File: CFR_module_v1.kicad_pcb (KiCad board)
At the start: 2 copper layers, 51 parts, among them J1 Conn_01x20, J2 Conn_01x20

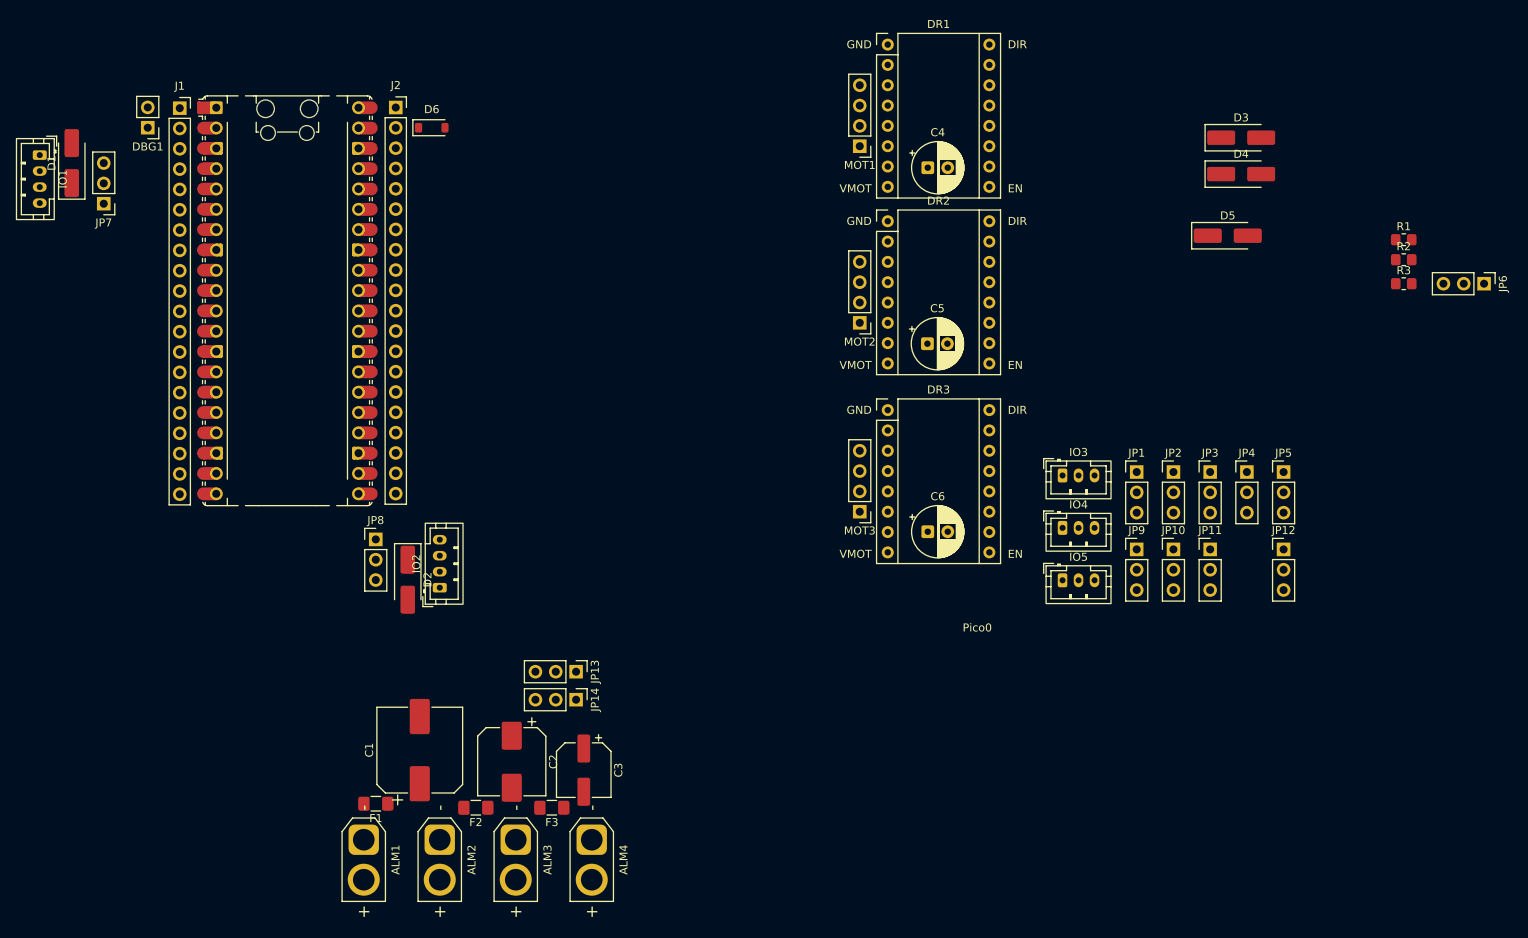
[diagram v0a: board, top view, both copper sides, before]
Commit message: pcb ok
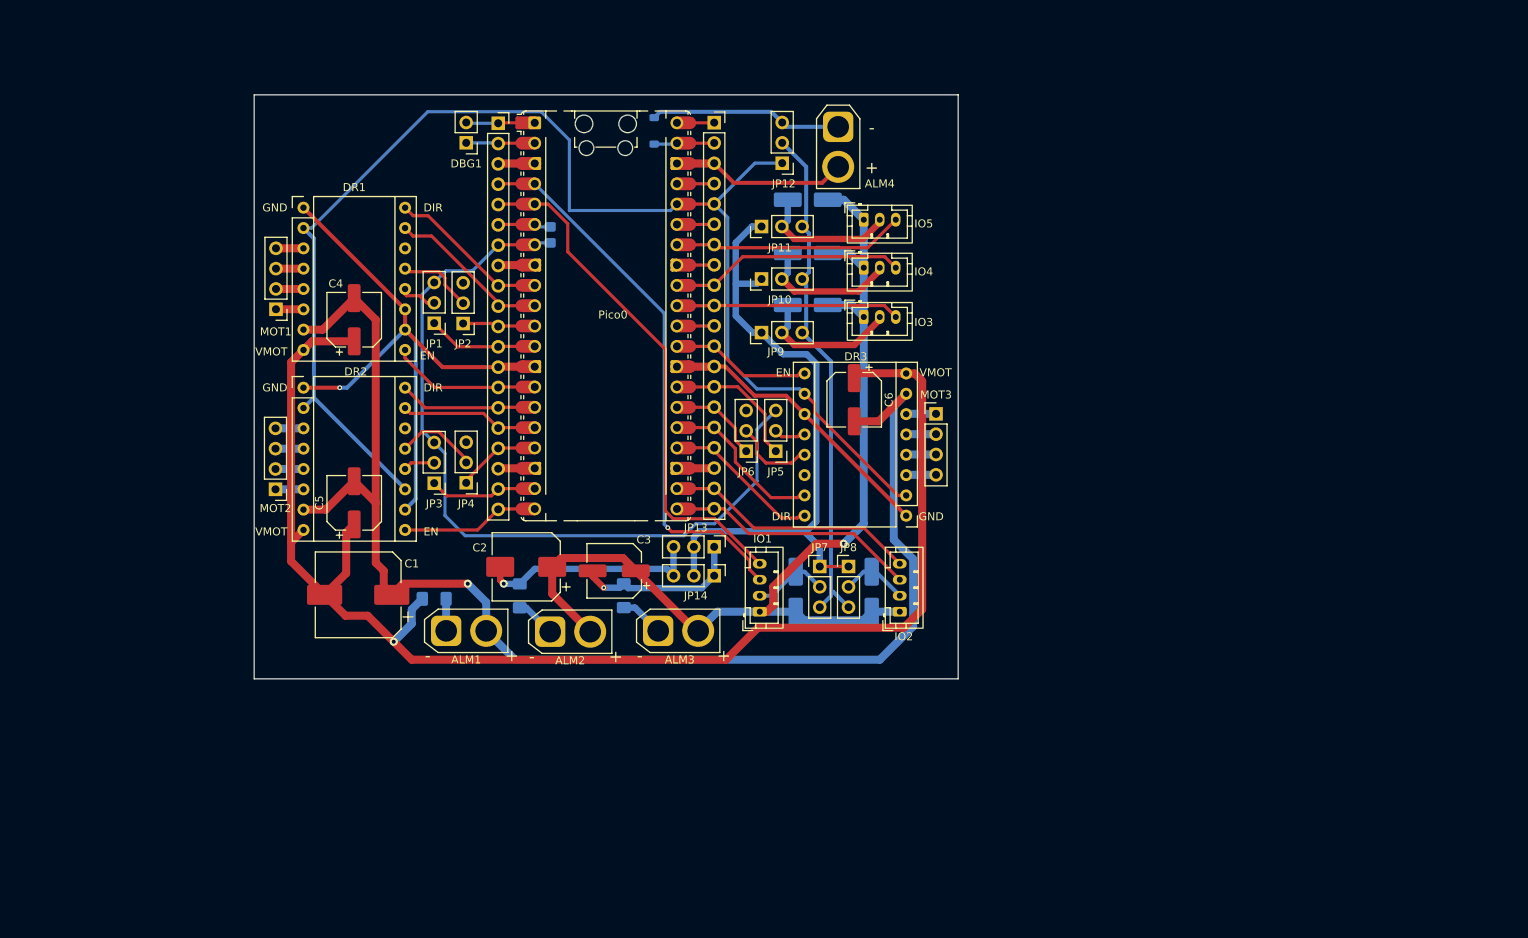
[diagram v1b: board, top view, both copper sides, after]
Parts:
- removed R2, R3: 1k, Resistor_SMD:R_0805_2012Metric_Pad1.20x1.40mm_HandSolder
- C4, C5, C6: footprint Capacitor_THT:CP_Radial_D6.3mm_P2.50mm -> Capacitor_SMD:CP_Elec_6.3x7.7
- D1, D2, D3, D4, D5, D6, F1, F2, F3, R1: moved to B.Cu
- moved R1 106.7 mm to (100.3, 83.4), turned to -90 degrees
- moved IO1 106.6 mm to (126.5, 130.5), turned to 90 degrees
- moved D1 105.2 mm to (131.0, 128.0), turned to -90 degrees
- moved JP7 100.3 mm to (134.0, 124.8), turned to 0 degrees
- moved JP4 97.6 mm to (89.8, 114.4), turned to 180 degrees
- moved JP3 97.0 mm to (85.8, 114.4), turned to 180 degrees
- moved JP6 94.6 mm to (124.8, 110.4), turned to 180 degrees
- moved ALM4 94.3 mm to (136.3, 69.9)
- moved JP2 90.7 mm to (89.4, 94.5), turned to 180 degrees
- moved JP1 89.8 mm to (85.8, 94.4), turned to 180 degrees
- moved JP12 79.1 mm to (129.3, 74.4), turned to 180 degrees
- moved DR2 75.9 mm to (69.5, 102.5)
- moved MOT2 75.9 mm to (66.0, 115.2)
- moved DR1 75.8 mm to (69.5, 80.0)
- moved MOT1 75.8 mm to (66.0, 92.7)
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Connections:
- ALM1 pad 2: GND -> GNDPWR1
- ALM2 pad 2: GND -> GNDPWR2
- ALM3 pad 2: GND -> GNDPWR2
- C1 pad 1: GND -> GNDPWR1
- C2 pad 1: GND -> GNDPWR2
- C3 pad 1: GND -> GNDPWR2
- C4 pad 2: GND -> GNDPWR1
- C5 pad 2: GND -> GNDPWR1
- C6 pad 2: GND -> GNDPWR1
- D1 pad 2: GND -> GNDPWR2
- D2 pad 2: GND -> GNDPWR2
- D3 pad 2: GND -> GNDPWR2
- D4 pad 2: GND -> GNDPWR2
- D5 pad 2: GND -> GNDPWR2
- DR1 pad 10: +3V3_Pico -> GND
- DR1 pad 7: GND -> GNDPWR1
- DR2 pad 10: +3V3_Pico -> GND
- DR2 pad 11: GND -> +3V3_Pico
- DR2 pad 7: GND -> GNDPWR1
- DR3 pad 15: GP21 -> GP19
- DR3 pad 16: GP22 -> GP18
- DR3 pad 7: GND -> GNDPWR1
- DR3 pad 9: GP18 -> GP22
- IO1 pad 1: GND -> GNDPWR2
- IO2 pad 1: GND -> GNDPWR2
- IO3 pad 1: GND -> GNDPWR2
- IO4 pad 1: GND -> GNDPWR2
- IO5 pad 1: GND -> GNDPWR2
- JP2 pad 3: GP4 -> unconnected-(JP2-B-Pad3)
- JP4 pad 3: GP4 -> unconnected-(JP4-B-Pad3)
- JP5 pad 1: GP19 -> GP21
- JP6 pad 3: GP4 -> unconnected-(JP6-B-Pad3)
- R1 pad 1: GP5 -> GP4
- R1 pad 2: GP4 -> GP5
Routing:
- net +BATT: track 0.00 -> 177.8 mm, vias 0 -> 1
- net GNDPWR1: track 0.00 -> 170.8 mm, vias 0 -> 1
- net +3V3_Pico: track 0.00 -> 168.5 mm
- net GND: track 0.00 -> 154.8 mm, vias 0 -> 1
- net GNDPWR2: track 0.00 -> 132.5 mm, vias 0 -> 1
- net GP5: track 0.00 -> 100.2 mm
- net +V2: track 0.00 -> 78.6 mm
- net GP2: track 0.00 -> 69.3 mm, vias 0 -> 1
- net +V1: track 0.00 -> 65.7 mm
- net GP3: track 0.00 -> 65.2 mm
- net GP17: track 0.00 -> 31.8 mm
- net GP16: track 0.00 -> 31.5 mm
- net GP27_A1: track 0.00 -> 29.4 mm
- net GP28_A2: track 0.00 -> 29.0 mm
- net +9V: track 0.00 -> 28.3 mm, vias 0 -> 1
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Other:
- board outline added: 88 x 73 mm

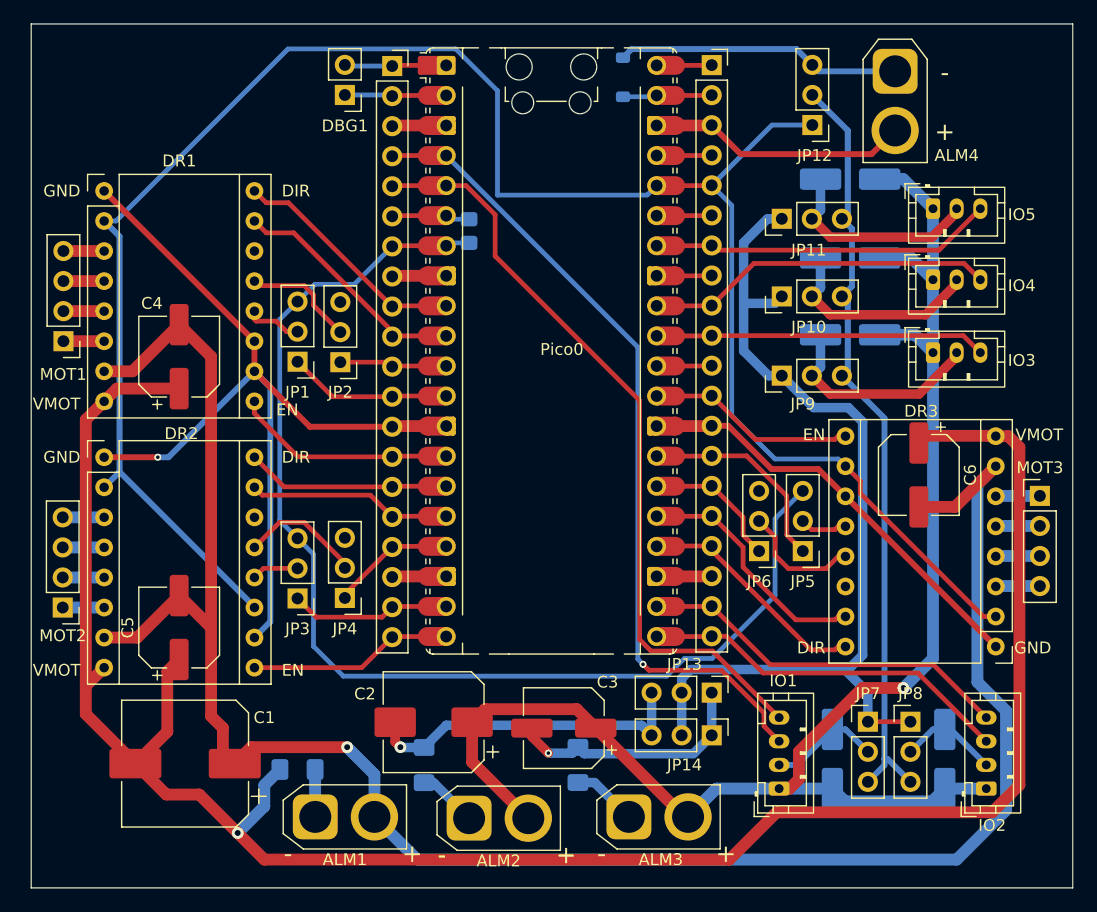
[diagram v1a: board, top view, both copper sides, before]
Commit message: fini avant modifs
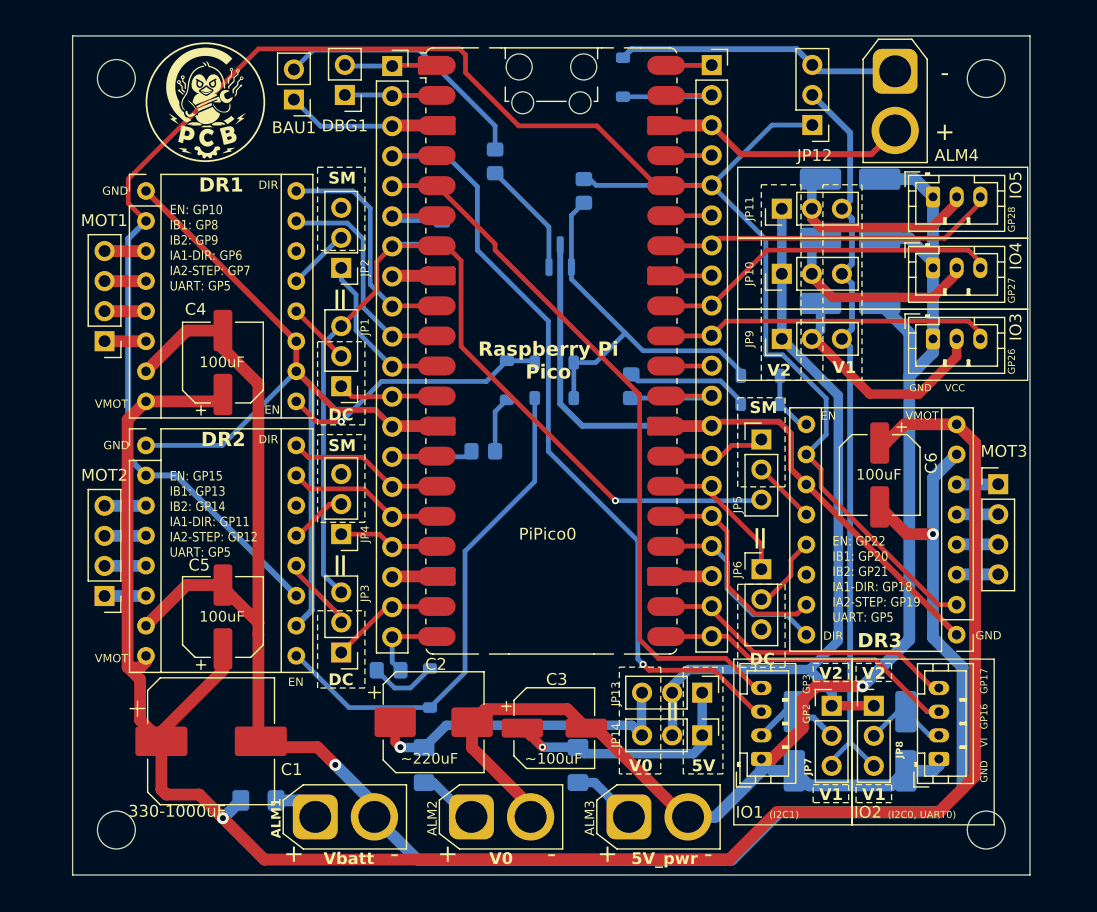
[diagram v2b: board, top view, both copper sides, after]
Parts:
- added BAU1: Conn_01x02, Connector_PinHeader_2.54mm:PinHeader_1x02_P2.54mm_Vertical, F.Cu at (85.5, 72.3)
- added D10: D_Schottky, Diode_SMD:D_SOD-123, B.Cu at (103.5, 96.0)
- added D11: D_Schottky, Diode_SMD:D_SOD-123, B.Cu at (97.0, 122.0)
- added D12: D_Schottky, Diode_SMD:D_SOD-123, B.Cu at (124.9, 98.0)
- added D7: D_Schottky, Diode_SMD:D_SOD-123, B.Cu at (107.5, 94.5)
- added D8: D_Schottky, Diode_SMD:D_SOD-123, B.Cu at (107.5, 97.5)
- added D9: D_Schottky, Diode_SMD:D_SOD-123, B.Cu at (124.9, 95.6)
- added G***: LOGO, Visuels_custom:logo_PCB, F.Cu at (78.2, 72.5)
- added H1: MountingHole, MountingHole:MountingHole_3.2mm_M3, F.Cu at (70.5, 70.5)
- added H2: MountingHole, MountingHole:MountingHole_3.2mm_M3, F.Cu at (144.0, 70.5)
- added H3: MountingHole, MountingHole:MountingHole_3.2mm_M3, F.Cu at (70.5, 134.0)
- added H4: MountingHole, MountingHole:MountingHole_3.2mm_M3, F.Cu at (144.0, 134.0)
- added Q1: NPN, Package_TO_SOT_SMD:SOT-23, B.Cu at (108.0, 85.5)
- added R2: 1k, Resistor_SMD:R_0805_2012Metric_Pad1.20x1.40mm_HandSolder, B.Cu at (102.5, 77.5)
- added R3: 10k, Resistor_SMD:R_0805_2012Metric_Pad1.20x1.40mm_HandSolder, B.Cu at (110.0, 80.0)
- added R4: 1k, Resistor_SMD:R_0805_2012Metric_Pad1.20x1.40mm_HandSolder, B.Cu at (101.5, 102.0)
- added R5: 1k, Resistor_SMD:R_0805_2012Metric_Pad1.20x1.40mm_HandSolder, B.Cu at (93.5, 120.5)
- added R6: 1k, Resistor_SMD:R_0805_2012Metric_Pad1.20x1.40mm_HandSolder, B.Cu at (114.0, 96.5)
- PiPico0: renamed from Pico0; footprint Module:RaspberryPi_Pico_Common_Unspecified -> Module:RaspberryPi_Pico_Common_SMD
- moved JP5 10.1 mm to (125.0, 101.0), turned to 0 degrees
- moved JP2 7.97 mm to (89.5, 86.5)
- moved JP3 5.88 mm to (89.5, 119.0)
- moved JP4 5.40 mm to (89.5, 109.0)
- moved IO2 4.72 mm to (140.0, 128.0)
- moved JP1 4.24 mm to (89.5, 96.5)
- moved F1 4.21 mm to (82.5, 131.5)
- moved C5 3.80 mm to (79.5, 116.0)
- moved C4 3.73 mm to (79.5, 94.5)
- moved DR2 3.67 mm to (73.0, 101.5)
- moved MOT2 3.66 mm to (69.5, 114.2)
- moved MOT3 3.66 mm to (145.0, 104.8)
- moved D2 3.62 mm to (137.2, 126.5)
- moved D1 3.55 mm to (127.8, 126.5)
- moved DR1 3.53 mm to (73.0, 80.0)
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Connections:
- C1 pad 1: GNDPWR1 -> +BATT
- C1 pad 2: +BATT -> GNDPWR1
- C2 pad 1: GNDPWR2 -> +9V
- C2 pad 2: +9V -> GNDPWR2
- C3 pad 1: GNDPWR2 -> +5V
- C3 pad 2: +5V -> GNDPWR2
- DR1 pad 9: GP10 -> M1_EN
- DR2 pad 9: GP15 -> M2_EN
- DR3 pad 9: GP22 -> M3_EN
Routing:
- net M2_EN: track 0.00 -> 42.9 mm
- net Net-(D7-A): track 0.00 -> 33.2 mm
- net GND: track 154.8 -> 184.4 mm, vias 1 -> 0
- net M1_EN: track 0.00 -> 23.1 mm, vias 0 -> 1
- net Net-(BAU1-Pin_2): track 0.00 -> 22.3 mm
- net GP5: track 100.2 -> 81.0 mm, vias 0 -> 1
- net +V2: track 78.6 -> 65.8 mm
- net GNDPWR1: track 170.8 -> 159.4 mm, vias 1 -> 2
- net +BATT: track 177.8 -> 167.3 mm
- net Net-(D12-A): track 0.00 -> 10.4 mm
- net Net-(Q1-B): track 0.00 -> 9.82 mm
- net GP15: track 17.3 -> 7.67 mm
- net GP21: track 17.6 -> 9.43 mm
- net GP10: track 18.8 -> 11.5 mm
- net GP22: track 17.6 -> 11.6 mm
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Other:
- board size 88 x 73 mm -> 80.9 x 70.9 mm
- board text added: "(I2C0, UART0)"
- board text added: "(I2C1)"
- board text added: "100uF"
- board text added: "10k"
- board text added: "1k"
- board text added: "330-1000uF"
- board text added: "5V"
- board text added: "5V_pwr"
- board text added: "="
- board text added: "DC"
- board text added: "EN: GP10 IB1: GP8 IB2: GP9 IA1-DIR: GP6 IA2-STEP: GP7 UART: GP5"
- board text added: "EN: GP15 IB1: GP13 IB2: GP14 IA1-DIR: GP11 IA2-STEP: GP12 UART: GP5"
- board text added: "EN: GP22 IB1: GP20 IB2: GP21 IA1-DIR: GP18 IA2-STEP: GP19 UART: GP5"
- board text added: "GND"
- board text added: "GP16"
- board text added: "GP17"
- board text added: "GP2"
- board text added: "GP26"
- board text added: "GP27"
- board text added: "GP28"
- board text added: "GP3"
- board text added: "Raspberry Pi Pico"
- board text added: "SM"
- board text added: "V0"
- board text added: "V1"
- board text added: "V2"
- board text added: "VCC"
- board text added: "VI"
- board text added: "Vbatt"
- board text added: "~100uF"
- board text added: "~220uF"
